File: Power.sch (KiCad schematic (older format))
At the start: 58 parts, among them J3 Conn_01x02, J4 Conn_01x02, J5 Conn_ARM_JTAG_SWD_10, Q1 MMBT5401LT1G, Q2 Q_NMOS_GDS, Q3 MMBT3904, Q4 Q_NMOS_GDS, Q5 Q_NMOS_GDS, Q6 Q_NMOS_GDS, U10 LMZ21700SIL, U6 LM5066, U7 STM32L011K4Tx, U8 ti-LM5163

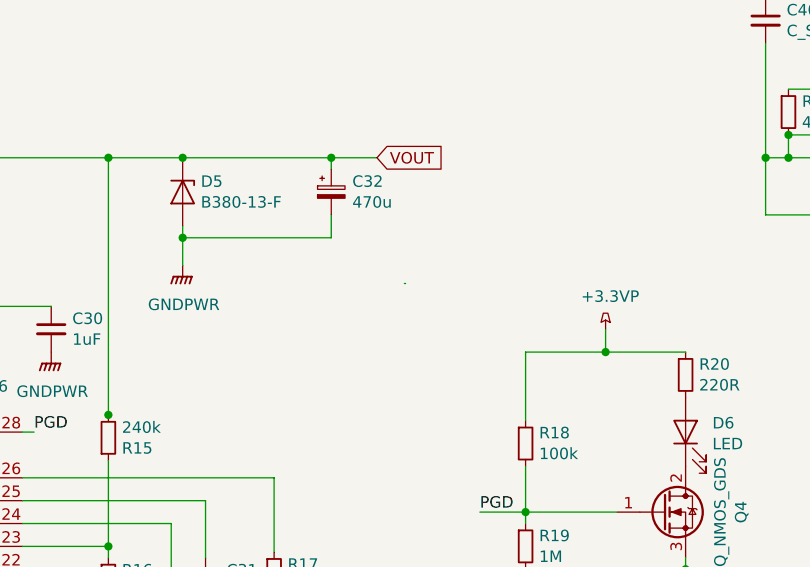
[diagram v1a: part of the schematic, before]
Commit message: Silk screen and cosmetic fixes
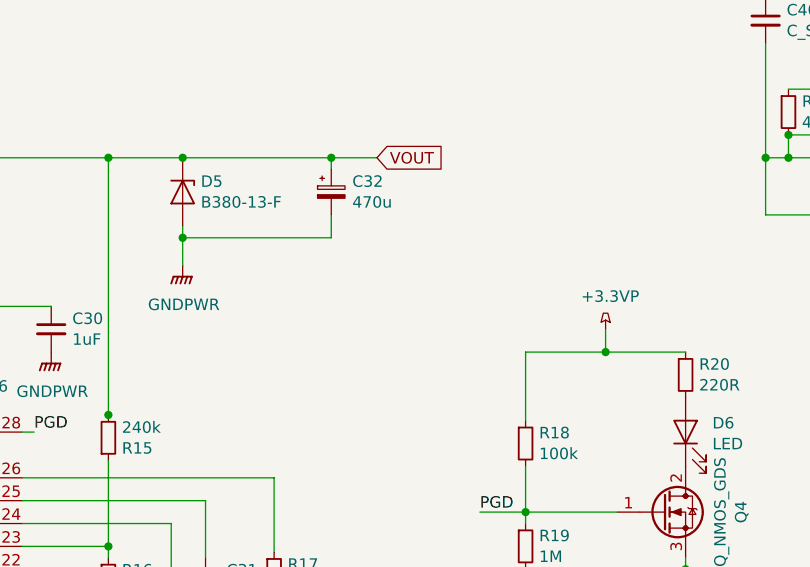
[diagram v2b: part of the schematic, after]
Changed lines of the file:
@@
 Wire Wire Line
 	10695 4600 10700 4600
-Wire Wire Line
-	8270 2100 8275 2100
 Connection ~ 9950 4000
 Connection ~ 10250 4600
